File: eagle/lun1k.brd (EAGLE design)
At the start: 127.6 x 60.4 mm, 102 parts, among them IC1 LTC3558, IC3 STM32F405RGT, IC4 NRF24L01SMD, J2 XF2-3015-1LW, Q1 Q12M-SMD-S, Q2 3.2X2.5CRYSTAL, SW1 JS102011SAQN, SW2 SWITCH_MCTAEF, SW3 SWITCH_MCTAEF, SW4 SWITCH_MCTAEF, T5 SI2301DS, T6 SI2301DS, U1 N35P112, X1 MICROUSB, X1_ JST-PH3

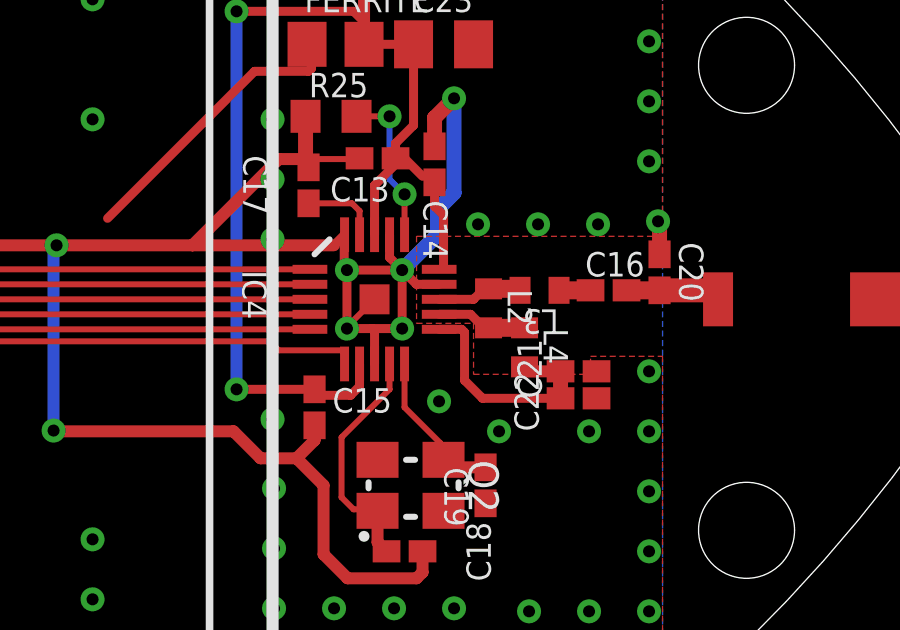
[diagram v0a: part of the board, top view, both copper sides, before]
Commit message: routing
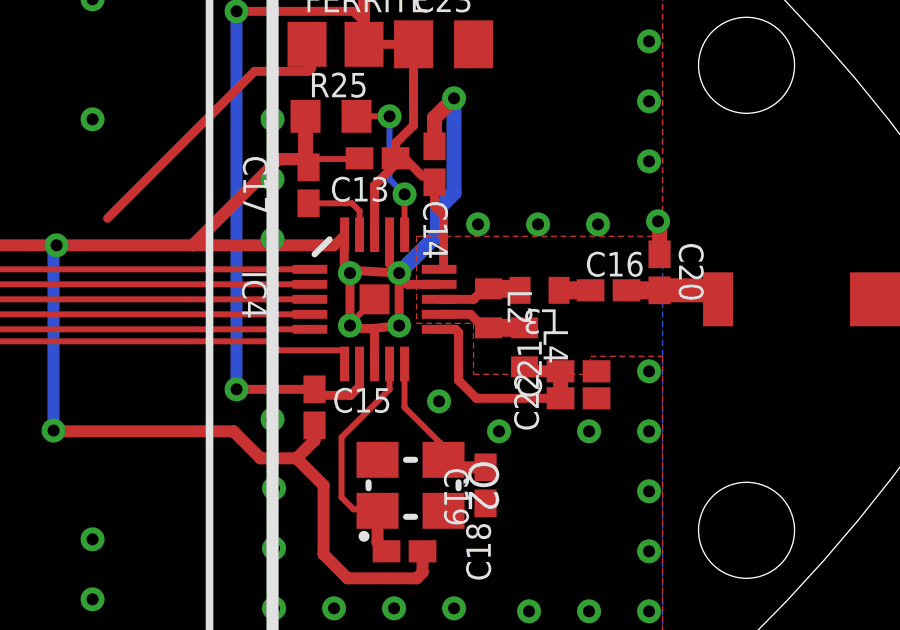
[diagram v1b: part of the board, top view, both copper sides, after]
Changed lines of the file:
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@@
 </class>
 </classes>
-<designrules name="default">
+<designrules name="default *">
 <description language="de">&lt;b&gt;EAGLE Design Rules&lt;/b&gt;
 &lt;p&gt;
@@
 <param name="mlMinCreamFrame" value="0mil"/>
 <param name="mlMaxCreamFrame" value="0mil"/>
-<param name="mlViaStopLimit" value="0.4mm"/>
+<param name="mlViaStopLimit" value="2.8mm"/>
 <param name="srRoundness" value="0"/>
 <param name="srMinRoundness" value="0mil"/>
@@
 <wire x1="41" y1="5.3" x2="36.3" y2="10" width="0.5" layer="16"/>
 <wire x1="36.3" y1="10" x2="36.3" y2="16" width="0.5" layer="16"/>
-<wire x1="0.6071" y1="24.2929" x2="0.6071" y2="22.9216" width="0" layer="19" extent="1-16"/>
-<wire x1="-0.3" y1="24.3" x2="0.6071" y2="24.2929" width="0" layer="19" extent="1-16"/>
 <wire x1="77.2217" y1="4.675" x2="78.6" y2="4.675" width="0.2" layer="1"/>
 <wire x1="78.3892" y1="2.154" x2="78.354" y2="2.154" width="0.2" layer="1"/>
@@
 <wire x1="68.8" y1="1.8" x2="68.7012" y2="1.7012" width="0.4" layer="16"/>
 <wire x1="60.5" y1="1.8" x2="68.8" y2="1.8" width="0.4" layer="1"/>
-<wire x1="78.3892" y1="2.154" x2="78.3892" y2="1.0658" width="0.3" layer="1"/>
-<wire x1="78.3892" y1="1.0658" x2="78.48" y2="0.975" width="0.2" layer="1"/>
-<wire x1="79.9" y1="1.395" x2="79.9" y2="2.154" width="0.3" layer="1"/>
-<wire x1="80.32" y1="0.975" x2="79.9" y2="1.395" width="0.3" layer="1"/>
-<wire x1="78.48" y1="0.975" x2="78.48" y2="-0.975" width="0.3" layer="1"/>
-<wire x1="78.48" y1="-0.975" x2="78.5065" y2="-0.975" width="0.2" layer="1"/>
+<wire x1="78.3892" y1="2.154" x2="78.3892" y2="0.9658" width="0.3" layer="1"/>
+<wire x1="78.3892" y1="0.9658" x2="78.58" y2="0.875" width="0.2" layer="1"/>
+<wire x1="79.9" y1="1.195" x2="79.9" y2="2.154" width="0.3" layer="1"/>
+<wire x1="80.22" y1="0.875" x2="79.9" y2="1.195" width="0.3" layer="1"/>
+<wire x1="78.58" y1="0.875" x2="78.58" y2="-0.875" width="0.3" layer="1"/>
+<wire x1="78.58" y1="-0.875" x2="78.5065" y2="-0.975" width="0.2" layer="1"/>
 <wire x1="78.5065" y1="-0.975" x2="79.32" y2="-0.975" width="0.3" layer="1"/>
-<wire x1="79.32" y1="-0.975" x2="80.32" y2="-0.975" width="0.3" layer="1"/>
-<wire x1="80.32" y1="-0.975" x2="80.32" y2="0.975" width="0.3" layer="1"/>
-<wire x1="80.32" y1="0.975" x2="78.515" y2="0.975" width="0.3" layer="1"/>
+<wire x1="79.32" y1="-0.975" x2="80.22" y2="-0.875" width="0.3" layer="1"/>
+<wire x1="80.22" y1="-0.875" x2="80.22" y2="0.875" width="0.3" layer="1"/>
+<wire x1="80.22" y1="0.875" x2="78.515" y2="0.975" width="0.3" layer="1"/>
 <wire x1="78.515" y1="0.975" x2="78.49" y2="1" width="0.2" layer="1"/>
-<wire x1="80.795" y1="0.5" x2="81.554" y2="0.5" width="0.3" layer="1"/>
-<wire x1="80.32" y1="0.975" x2="80.795" y2="0.5" width="0.3" layer="1"/>
+<wire x1="80.495" y1="0.5" x2="81.554" y2="0.5" width="0.3" layer="1"/>
+<wire x1="80.22" y1="0.875" x2="80.495" y2="0.5" width="0.3" layer="1"/>
 <wire x1="79.4" y1="-1.055" x2="79.4" y2="-2.154" width="0.3" layer="1"/>
 <wire x1="79.32" y1="-0.975" x2="79.4" y2="-1.055" width="0.2" layer="1"/>
@@
 <wire x1="77.2" y1="4.4" x2="77.1" y2="4.5" width="0.5" layer="1"/>
 <wire x1="77.1" y1="4.5" x2="77.1" y2="6.1" width="0.5" layer="1"/>
-<wire x1="-4.2" y1="24.8" x2="15.2" y2="19.4" width="0" layer="19" extent="1-16"/>
-<wire x1="-3.5" y1="24" x2="-4.2" y2="24.8" width="0" layer="19" extent="1-16"/>
-<wire x1="-0.6" y1="24" x2="-3.5" y2="24" width="0" layer="19" extent="1-16"/>
-<wire x1="-0.3" y1="24.3" x2="-0.6" y2="24" width="0" layer="19" extent="1-16"/>
 <wire x1="88.9" y1="1.5" x2="88.9" y2="2.45" width="0.5" layer="1"/>
 <wire x1="88.9" y1="2.45" x2="88.85" y2="2.6" width="0.5" layer="1"/>
@@
 <wire x1="81.5" y1="3" x2="82.05" y2="3.55" width="0.5" layer="16"/>
 <wire x1="81.5" y1="2.155" x2="81.5" y2="3" width="0.5" layer="16"/>
-<wire x1="80.32" y1="0.975" x2="81.5" y2="2.155" width="0.5" layer="16"/>
+<wire x1="80.22" y1="0.875" x2="81.5" y2="2.155" width="0.5" layer="16"/>
 <wire x1="75.6" y1="-5.3" x2="76.8" y2="-5.3" width="0.4" layer="1"/>
 <wire x1="76.8" y1="-5.3" x2="77.4" y2="-4.7" width="0.4" layer="1"/>
@@
 <wire x1="76.8" y1="-5.3" x2="77.7" y2="-6.2" width="0.4" layer="1"/>
 <via x="36.4" y="16.1" extent="1-16" drill="0.4" shape="octagon"/>
-<via x="78.48" y="-0.975" extent="1-16" drill="0.4" shape="octagon" alwaysstop="yes"/>
-<via x="80.32" y="-0.975" extent="1-16" drill="0.4" shape="octagon" alwaysstop="yes"/>
+<via x="78.58" y="-0.875" extent="1-16" drill="0.4" shape="octagon" alwaysstop="yes"/>
+<via x="80.22" y="-0.875" extent="1-16" drill="0.4" shape="octagon" alwaysstop="yes"/>
 <via x="68.7012" y="-4.375" extent="1-16" drill="0.4" shape="octagon"/>
 <via x="68.8" y="1.8" extent="1-16" drill="0.4" shape="octagon"/>
-<via x="78.48" y="0.975" extent="1-16" drill="0.4" shape="octagon" alwaysstop="yes"/>
-<via x="80.32" y="0.975" extent="1-16" drill="0.4" shape="octagon" alwaysstop="yes"/>
+<via x="78.58" y="0.875" extent="1-16" drill="0.4" shape="octagon" alwaysstop="yes"/>
+<via x="80.22" y="0.875" extent="1-16" drill="0.4" shape="octagon" alwaysstop="yes"/>
 <via x="88.55" y="-4.4" extent="1-16" drill="0.4" shape="octagon"/>
 <via x="62.4" y="-4.5" extent="1-16" drill="0.4" shape="octagon"/>
@@
 <wire x1="85.6" y1="-2.4" x2="84.45" y2="-2.4" width="0.4" layer="1"/>
 <wire x1="84.45" y1="-2.4" x2="84.4" y2="-2.25" width="0.3" layer="1"/>
-<wire x1="82.3" y1="-1" x2="81.554" y2="-1" width="0.3" layer="1"/>
-<wire x1="82.4" y1="-1.1" x2="82.3" y2="-1" width="0.3" layer="1"/>
-<wire x1="82.4" y1="-2.7" x2="82.4" y2="-1.1" width="0.3" layer="1"/>
-<wire x1="83" y1="-3.3" x2="82.4" y2="-2.7" width="0.3" layer="1"/>
-<wire x1="83" y1="-3.3" x2="85.6" y2="-3.3" width="0.3" layer="1"/>
+<wire x1="82.1" y1="-1" x2="81.554" y2="-1" width="0.3" layer="1"/>
+<wire x1="82.2" y1="-1.1" x2="82.1" y2="-1" width="0.3" layer="1"/>
+<wire x1="82.2" y1="-2.7" x2="82.2" y2="-1.1" width="0.3" layer="1"/>
+<wire x1="82.8" y1="-3.3" x2="82.2" y2="-2.7" width="0.3" layer="1"/>
+<wire x1="82.8" y1="-3.3" x2="85.6" y2="-3.3" width="0.3" layer="1"/>
 </signal>
 <signal name="N$78">
@@
 <contactref element="U$2" pad="1"/>
 <contactref element="U$2" pad="1@1"/>
-<wire x1="-8.6565" y1="18.69" x2="-18.9435" y2="18.69" width="0" layer="19" extent="1-1"/>
-<wire x1="-8.6565" y1="-18.69" x2="-18.9435" y2="18.69" width="0" layer="19" extent="1-1"/>
-<wire x1="-18.9435" y1="-18.69" x2="-8.6565" y2="-18.69" width="0" layer="19" extent="1-1"/>
+<wire x1="-8.6565" y1="-18.69" x2="-18.9435" y2="-18.69" width="0" layer="19" extent="16-16"/>
+<wire x1="-8.6565" y1="18.69" x2="-8.6565" y2="-18.69" width="0" layer="19" extent="16-16"/>
+<wire x1="-18.9435" y1="18.69" x2="-8.6565" y2="18.69" width="0" layer="19" extent="16-16"/>
 </signal>
 <signal name="2">
@@
 <contactref element="U$2" pad="2"/>
 <contactref element="U$2" pad="2@1"/>
-<wire x1="-8.6565" y1="21.23" x2="-18.9435" y2="21.23" width="0" layer="19" extent="1-1"/>
-<wire x1="-8.6565" y1="-21.23" x2="-18.9435" y2="21.23" width="0" layer="19" extent="1-1"/>
-<wire x1="-18.9435" y1="-21.23" x2="-8.6565" y2="-21.23" width="0" layer="19" extent="1-1"/>
+<wire x1="-8.6565" y1="-21.23" x2="-18.9435" y2="-21.23" width="0" layer="19" extent="16-16"/>
+<wire x1="-8.6565" y1="21.23" x2="-8.6565" y2="-21.23" width="0" layer="19" extent="16-16"/>
+<wire x1="-18.9435" y1="21.23" x2="-8.6565" y2="21.23" width="0" layer="19" extent="16-16"/>
 </signal>
 <signal name="3">
@@
 <contactref element="U$2" pad="3"/>
 <contactref element="U$2" pad="3@1"/>
-<wire x1="-8.6565" y1="23.77" x2="-18.9435" y2="23.77" width="0" layer="19" extent="1-1"/>
-<wire x1="-8.6565" y1="-23.77" x2="-18.9435" y2="23.77" width="0" layer="19" extent="1-1"/>
-<wire x1="-18.9435" y1="-23.77" x2="-8.6565" y2="-23.77" width="0" layer="19" extent="1-1"/>
+<wire x1="-8.6565" y1="-23.77" x2="-18.9435" y2="-23.77" width="0" layer="19" extent="16-16"/>
+<wire x1="-8.6565" y1="23.77" x2="-8.6565" y2="-23.77" width="0" layer="19" extent="16-16"/>
+<wire x1="-18.9435" y1="23.77" x2="-8.6565" y2="23.77" width="0" layer="19" extent="16-16"/>
 </signal>
 <signal name="4">
@@
 <contactref element="U$2" pad="4"/>
 <contactref element="U$2" pad="4@1"/>
-<wire x1="-8.6565" y1="26.31" x2="-18.9435" y2="26.31" width="0" layer="19" extent="1-1"/>
-<wire x1="-8.6565" y1="-26.31" x2="-18.9435" y2="26.31" width="0" layer="19" extent="1-1"/>
-<wire x1="-18.9435" y1="-26.31" x2="-8.6565" y2="-26.31" width="0" layer="19" extent="1-1"/>
+<wire x1="-8.6565" y1="-26.31" x2="-18.9435" y2="-26.31" width="0" layer="19" extent="16-16"/>
+<wire x1="-8.6565" y1="26.31" x2="-8.6565" y2="-26.31" width="0" layer="19" extent="16-16"/>
+<wire x1="-18.9435" y1="26.31" x2="-8.6565" y2="26.31" width="0" layer="19" extent="16-16"/>
 </signal>
 </signals>
